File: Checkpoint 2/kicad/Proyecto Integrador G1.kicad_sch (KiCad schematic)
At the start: 50 parts, among them J1 Conn_01x02, J2 Conn_01x02, Q1 BC547, Q10 BC547, Q2 BC547, Q3 BC547, Q4 BC547, Q5 BC557, Q6 BC557, Q7 BC547, Q8 TIP42C, Q9 BC547, U1 TL431LP, U2 LM358

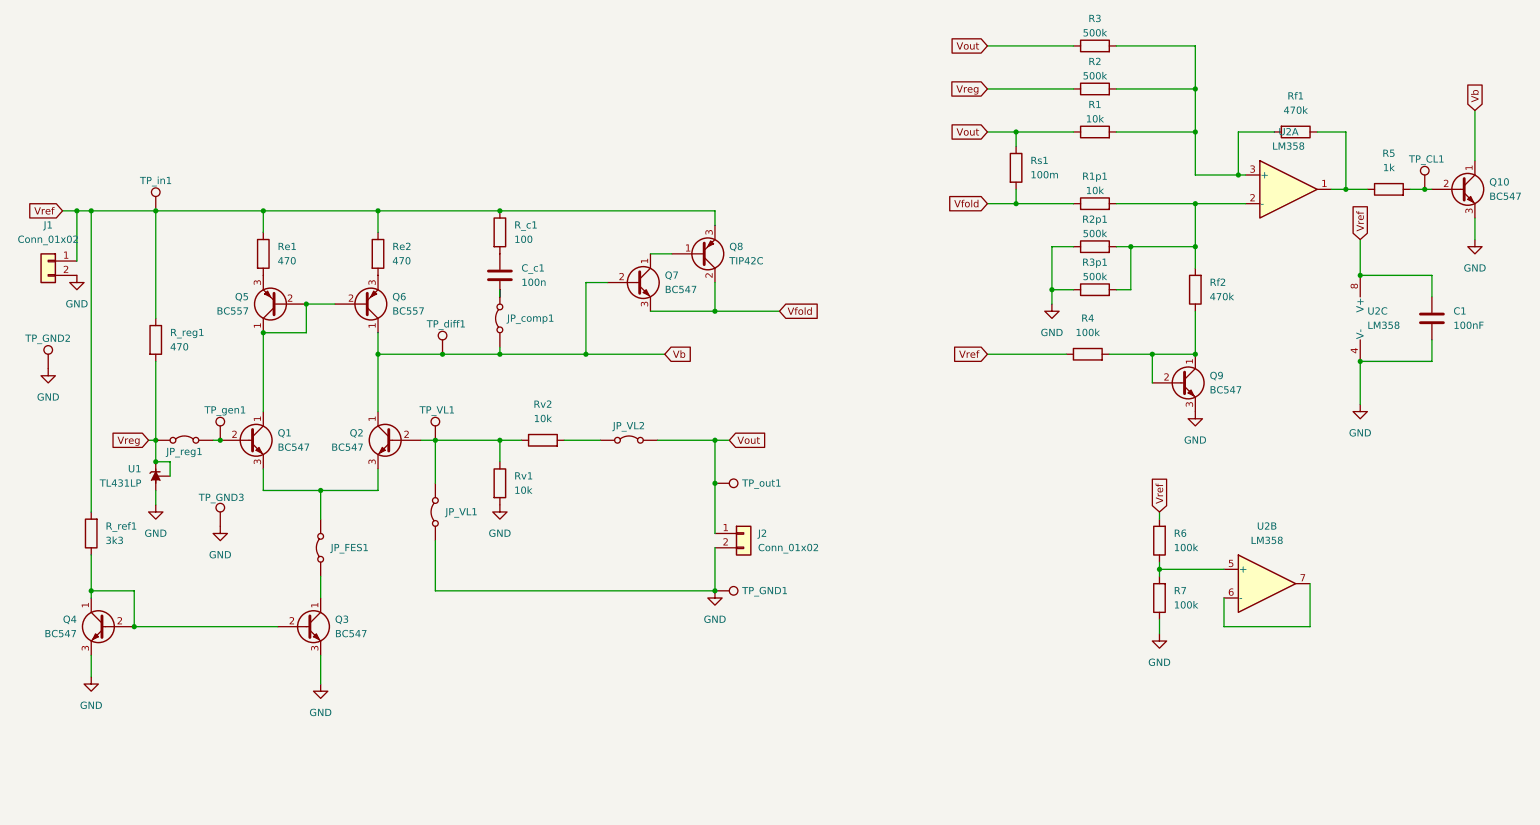
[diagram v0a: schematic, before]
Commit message: rev 1.1
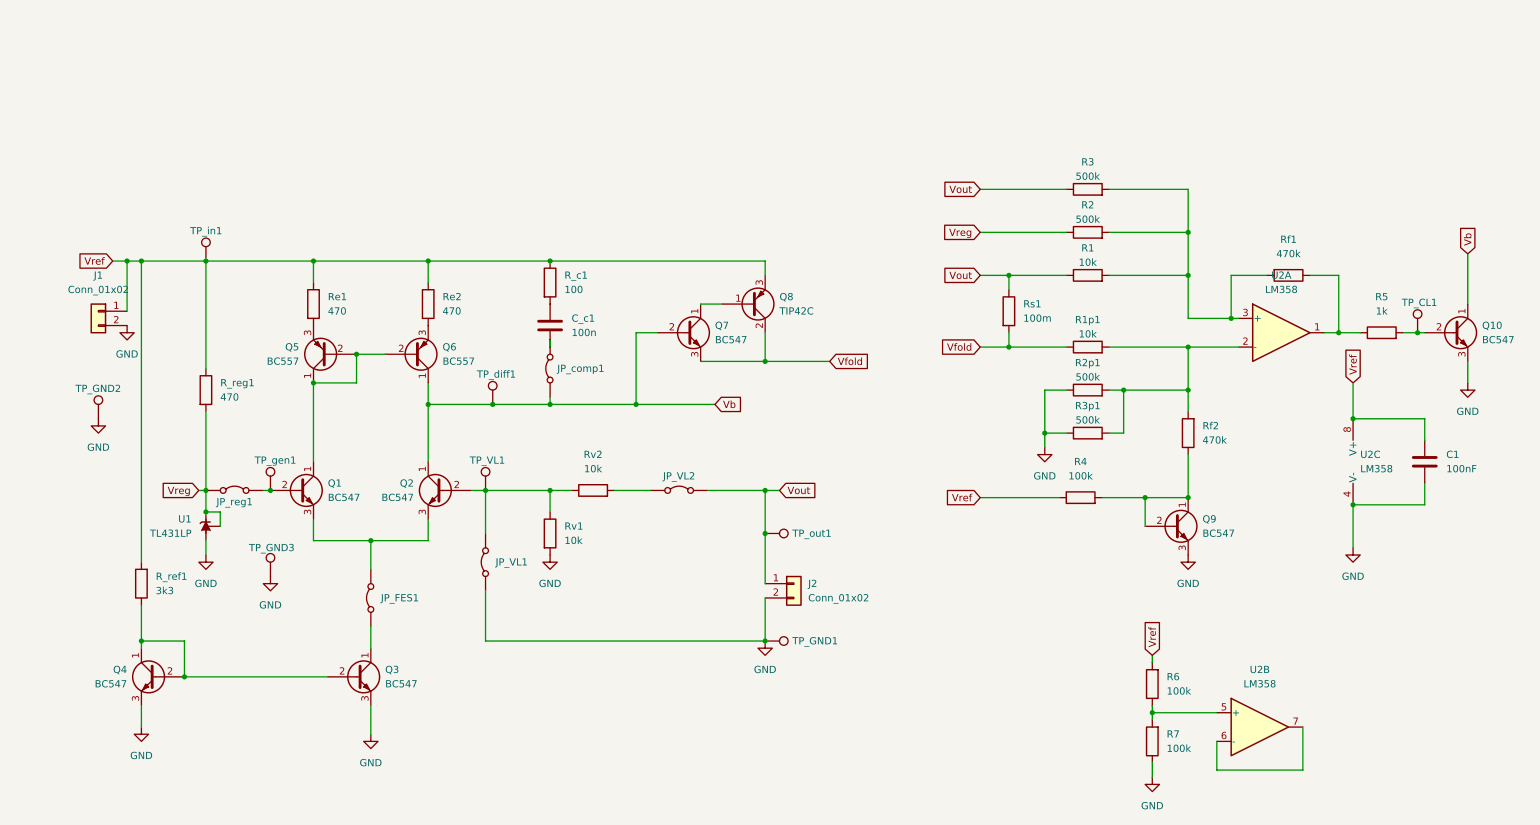
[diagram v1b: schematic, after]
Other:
- moved on the sheet: C1, C_c1, J1, J2, JP_FES1, JP_VL1, JP_VL2, JP_comp1, JP_reg1, Q1, Q10, Q2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
